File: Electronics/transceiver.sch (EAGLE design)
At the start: 8 parts, among them U1 MCP2515, U2 MCP2551

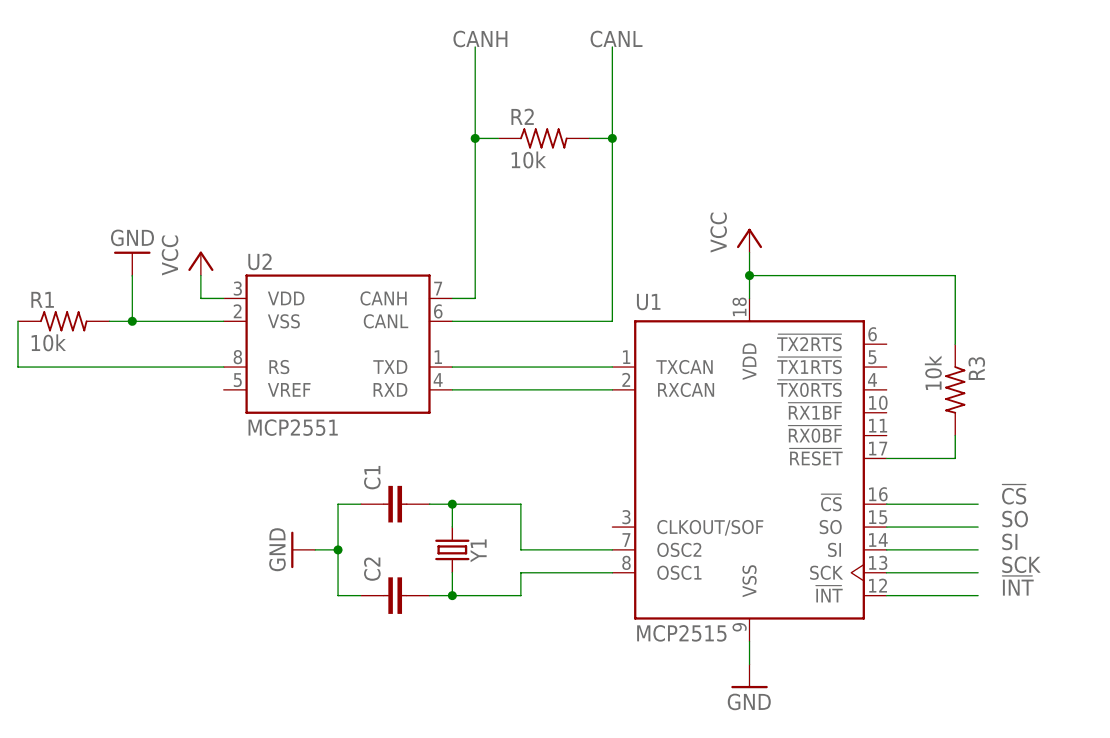
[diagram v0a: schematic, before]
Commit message: Fix merge conflict
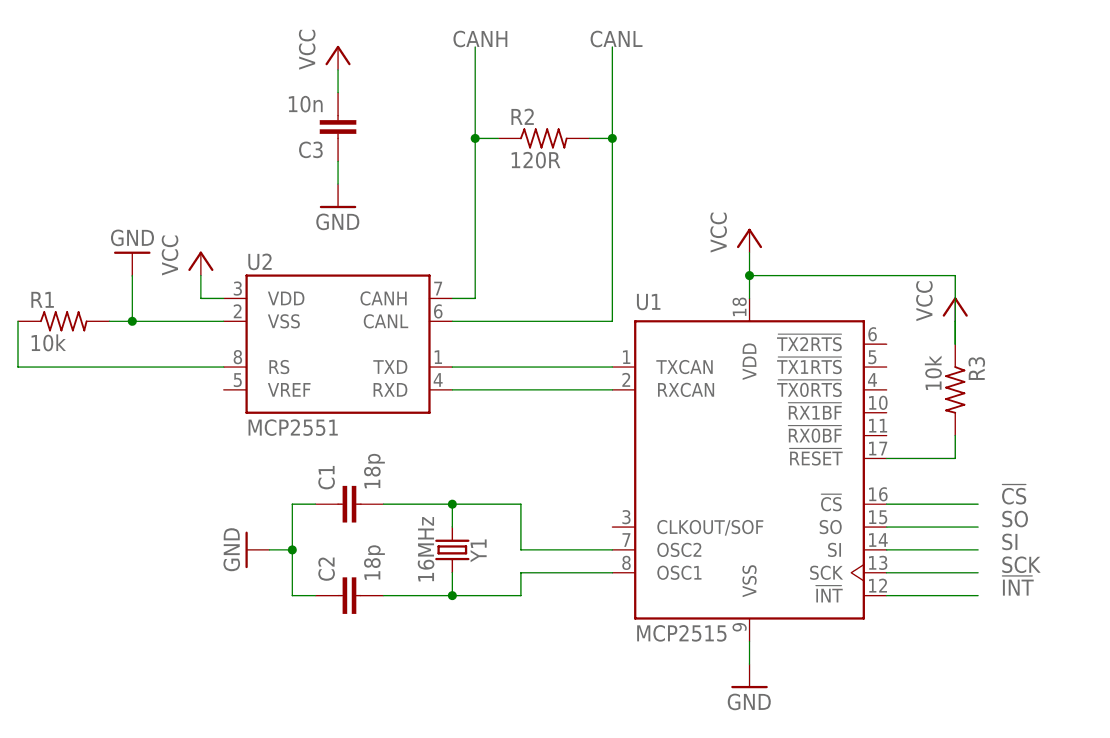
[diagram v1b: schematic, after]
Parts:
- added C3: 10n, rcl:C-EU025-030X050
- C1, C2: value (none) -> 18p
- R2: value 10k -> 120R
- Y1: value (none) -> 16MHz
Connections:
- net GND: now also C3.1
- net VCC: now also C3.2
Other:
- moved on the sheet: C1, C2
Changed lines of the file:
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@@
 <?xml version="1.0" encoding="utf-8"?>
 <!DOCTYPE eagle SYSTEM "eagle.dtd">
-<eagle version="8.0.0">
+<eagle version="8.1.0">
 <drawing>
 <settings>
@@
 <setting verticaltext="up"/>
 </settings>
-<grid distance="0.1" unitdist="inch" unit="inch" style="lines" multiple="1" display="yes" altdistance="0.01" altunitdist="inch" altunit="inch"/>
+<grid distance="0.1" unitdist="inch" unit="inch" style="lines" multiple="1" display="no" altdistance="0.01" altunitdist="inch" altunit="inch"/>
 <layers>
 <layer number="1" name="Top" color="4" fill="1" visible="no" active="no"/>
@@
 <part name="P+1" library="supply1" deviceset="VCC" device=""/>
 <part name="R1" library="rcl" deviceset="R-US_" device="0204/7" value="10k"/>
-<part name="R2" library="rcl" deviceset="R-US_" device="0204/7" value="10k"/>
-<part name="Y1" library="SparkFun-Clocks" deviceset="CRYSTAL" device="PTH-HC49UV"/>
-<part name="C1" library="rcl" deviceset="C-EU" device="025-030X050"/>
-<part name="C2" library="rcl" deviceset="C-EU" device="025-030X050"/>
+<part name="R2" library="rcl" deviceset="R-US_" device="0204/7" value="120R"/>
+<part name="Y1" library="SparkFun-Clocks" deviceset="CRYSTAL" device="PTH-HC49UV" value="16MHz"/>
+<part name="C1" library="rcl" deviceset="C-EU" device="025-030X050" value="18p"/>
+<part name="C2" library="rcl" deviceset="C-EU" device="025-030X050" value="18p"/>
 <part name="GND3" library="supply1" deviceset="GND" device=""/>
 <part name="R3" library="rcl" deviceset="R-US_" device="0204/7" value="10k"/>
+<part name="C3" library="rcl" deviceset="C-EU" device="025-030X050" value="10n"/>
+<part name="GND5" library="supply1" deviceset="GND" device=""/>
+<part name="P+3" library="supply1" deviceset="VCC" device=""/>
+<part name="P+4" library="supply1" deviceset="VCC" device=""/>
 </parts>
 <sheets>
@@
 <instance part="R2" gate="G$1" x="22.86" y="22.86"/>
 <instance part="Y1" gate="G$1" x="12.7" y="-22.86" rot="R270"/>
-<instance part="C1" gate="G$1" x="5.08" y="-17.78" rot="R90"/>
-<instance part="C2" gate="G$1" x="5.08" y="-27.94" rot="R90"/>
-<instance part="GND3" gate="1" x="-5.08" y="-22.86" rot="R270"/>
+<instance part="C1" gate="G$1" x="0" y="-17.78" rot="R90"/>
+<instance part="C2" gate="G$1" x="0" y="-27.94" rot="R90"/>
+<instance part="GND3" gate="1" x="-10.16" y="-22.86" rot="R270"/>
 <instance part="R3" gate="G$1" x="68.58" y="-5.08" rot="R270"/>
+<instance part="C3" gate="G$1" x="0" y="22.86" rot="R180"/>
+<instance part="GND5" gate="1" x="0" y="15.24"/>
+<instance part="P+3" gate="VCC" x="0" y="33.02"/>
+<instance part="P+4" gate="VCC" x="68.58" y="5.08"/>
 </instances>
 <busses>
@@
 <wire x1="-15.24" y1="5.08" x2="-12.7" y2="5.08" width="0.1524" layer="91"/>
 </segment>
+<segment>
+<pinref part="P+3" gate="VCC" pin="VCC"/>
+<pinref part="C3" gate="G$1" pin="2"/>
+<wire x1="0" y1="30.48" x2="0" y2="27.94" width="0.1524" layer="91"/>
+</segment>
+<segment>
+<pinref part="R3" gate="G$1" pin="1"/>
+<wire x1="68.58" y1="0" x2="68.58" y2="2.54" width="0.1524" layer="91"/>
+<pinref part="P+4" gate="VCC" pin="VCC"/>
+</segment>
 </net>
 <net name="GND" class="0">
@@
 <segment>
 <pinref part="C1" gate="G$1" pin="1"/>
-<wire x1="2.54" y1="-17.78" x2="0" y2="-17.78" width="0.1524" layer="91"/>
-<wire x1="0" y1="-17.78" x2="0" y2="-22.86" width="0.1524" layer="91"/>
+<wire x1="-2.54" y1="-17.78" x2="-5.08" y2="-17.78" width="0.1524" layer="91"/>
+<wire x1="-5.08" y1="-17.78" x2="-5.08" y2="-22.86" width="0.1524" layer="91"/>
 <pinref part="C2" gate="G$1" pin="1"/>
-<wire x1="0" y1="-22.86" x2="0" y2="-27.94" width="0.1524" layer="91"/>
-<wire x1="0" y1="-27.94" x2="2.54" y2="-27.94" width="0.1524" layer="91"/>
+<wire x1="-5.08" y1="-22.86" x2="-5.08" y2="-27.94" width="0.1524" layer="91"/>
+<wire x1="-5.08" y1="-27.94" x2="-2.54" y2="-27.94" width="0.1524" layer="91"/>
 <pinref part="GND3" gate="1" pin="GND"/>
-<wire x1="0" y1="-22.86" x2="-2.54" y2="-22.86" width="0.1524" layer="91"/>
-<junction x="0" y="-22.86"/>
+<wire x1="-5.08" y1="-22.86" x2="-7.62" y2="-22.86" width="0.1524" layer="91"/>
+<junction x="-5.08" y="-22.86"/>
+</segment>
+<segment>
+<pinref part="C3" gate="G$1" pin="1"/>
+<pinref part="GND5" gate="1" pin="GND"/>
+<wire x1="0" y1="20.32" x2="0" y2="17.78" width="0.1524" layer="91"/>
 </segment>
 </net>
@@
 <wire x1="20.32" y1="-22.86" x2="30.48" y2="-22.86" width="0.1524" layer="91"/>
 <pinref part="C1" gate="G$1" pin="2"/>
-<wire x1="10.16" y1="-17.78" x2="12.7" y2="-17.78" width="0.1524" layer="91"/>
+<wire x1="5.08" y1="-17.78" x2="12.7" y2="-17.78" width="0.1524" layer="91"/>
 <junction x="12.7" y="-17.78"/>
 </segment>
@@
 <wire x1="12.7" y1="-27.94" x2="12.7" y2="-25.4" width="0.1524" layer="91"/>
 <pinref part="C2" gate="G$1" pin="2"/>
-<wire x1="10.16" y1="-27.94" x2="12.7" y2="-27.94" width="0.1524" layer="91"/>
+<wire x1="5.08" y1="-27.94" x2="12.7" y2="-27.94" width="0.1524" layer="91"/>
 <junction x="12.7" y="-27.94"/>
 </segment>
